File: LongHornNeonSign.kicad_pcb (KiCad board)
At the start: 2 copper layers, 68.1 x 76.2 mm, 19 parts, among them Q1 IRLZ44N, Q2 IRLZ44N, Q3 IRLZ44N

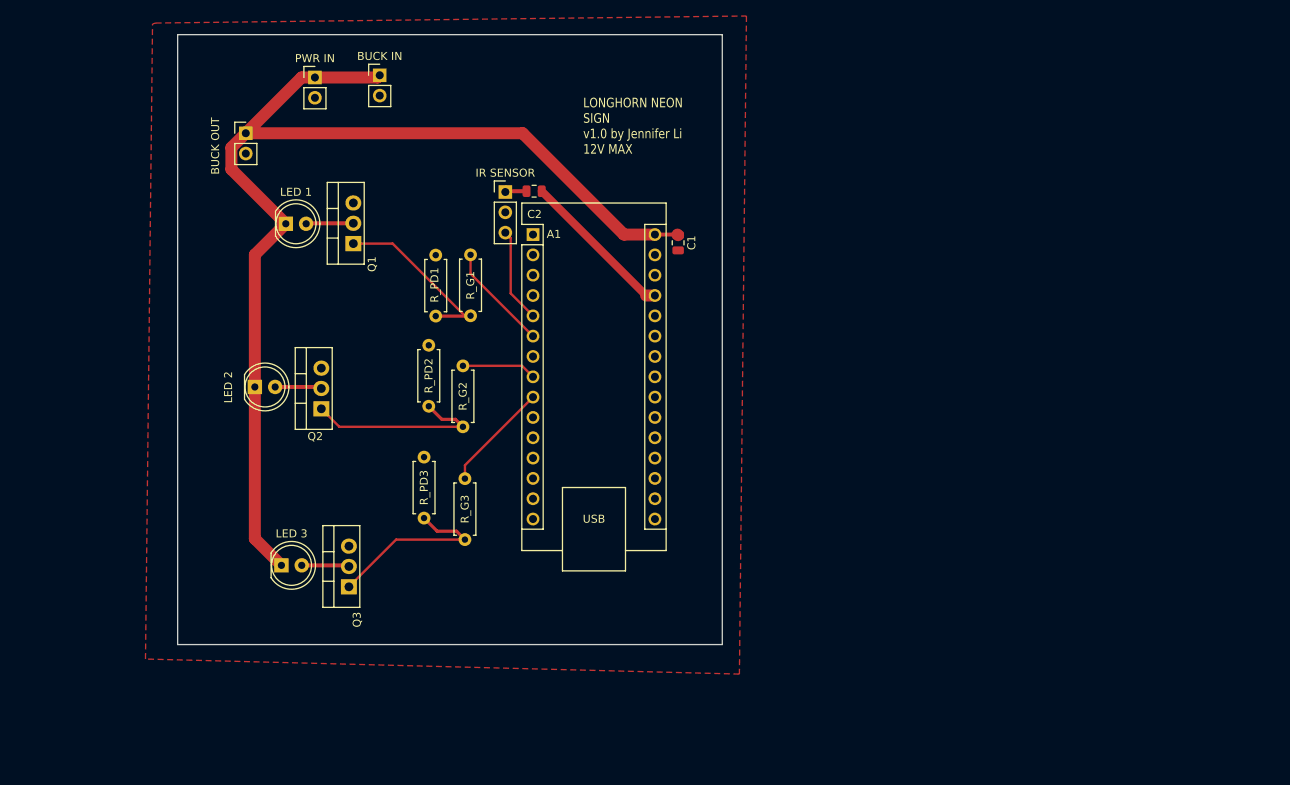
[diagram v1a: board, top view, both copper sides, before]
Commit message: update
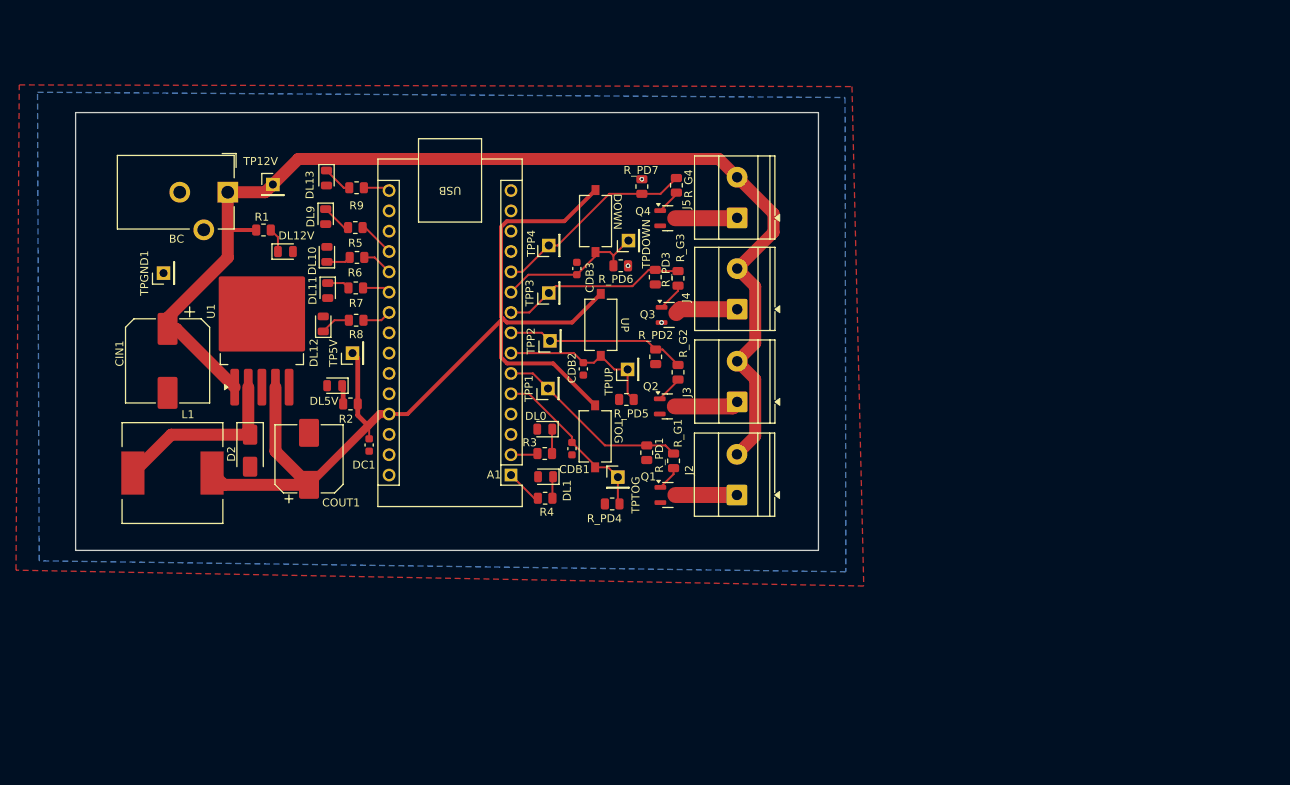
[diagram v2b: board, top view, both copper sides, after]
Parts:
- removed BUCK IN: Conn_01x02_Pin, Connector_PinHeader_2.54mm:PinHeader_1x02_P2.54mm_Vertical
- removed BUCK OUT: Conn_01x02_Pin, Connector_PinHeader_2.54mm:PinHeader_1x02_P2.54mm_Vertical
- removed C1, C2: 0.1uF, Capacitor_SMD:C_0805_2012Metric
- removed IR SENSOR: Conn_01x03, Connector_PinHeader_2.54mm:PinHeader_1x03_P2.54mm_Vertical
- removed LED 1: Conn_01x02_Pin, LED_THT:LED_D5.0mm
- removed LED 2: Conn_01x02_Pin, LED_THT:LED_D5.0mm
- removed LED 3: Conn_01x02_Pin, LED_THT:LED_D5.0mm
- removed PWR IN: Conn_01x02_Pin, Connector_PinHeader_2.54mm:PinHeader_1x02_P2.54mm_Vertical
- added BC: Barrel_Jack, Connector_BarrelJack:BarrelJack_CUI_PJ-102AH_Horizontal, F.Cu at (76.2, 71.6)
- added CDB1: 0.1uF, Capacitor_SMD:C_0603_1608Metric, F.Cu at (119.2, 103.7)
- added CDB2: 0.1uF, Capacitor_SMD:C_0603_1608Metric, F.Cu at (120.7, 93.7)
- added CDB3: 0.1uF, Capacitor_SMD:C_0603_1608Metric, F.Cu at (119.8, 81.2)
- added CIN1: 680μF, Capacitor_SMD:CP_Elec_10x10, F.Cu at (68.7, 92.7)
- added COUT1: 220μF, Capacitor_SMD:CP_Elec_8x10, F.Cu at (86.4, 105.0)
- added D2: SS34, Diode_SMD:D_SMA, F.Cu at (79.0, 103.9)
- added DC1: 0.1uF, Capacitor_SMD:C_0603_1608Metric, F.Cu at (93.9, 103.2)
- added DL0: DL_D0, LED_SMD:LED_0805_2012Metric, F.Cu at (115.8, 101.2)
- added DL1: DL_D1, LED_SMD:LED_0805_2012Metric, F.Cu at (115.9, 107.2)
- added DL10: DL_D10, LED_SMD:LED_0805_2012Metric, F.Cu at (88.6, 79.4)
- added DL11: DL_D11, LED_SMD:LED_0805_2012Metric, F.Cu at (88.7, 83.9)
- added DL12: DL_D12, LED_SMD:LED_0805_2012Metric, F.Cu at (88.1, 88.1)
- added DL12V: DL_12V, LED_SMD:LED_0805_2012Metric, F.Cu at (83.4, 79.0)
- added DL13: DL_D13, LED_SMD:LED_0805_2012Metric, F.Cu at (88.5, 69.8)
- added DL5V: DL_5V, LED_SMD:LED_0805_2012Metric, F.Cu at (89.6, 95.8)
- added DL9: DL_D9, LED_SMD:LED_0805_2012Metric, F.Cu at (88.4, 74.7)
- added DOWN: SW_Push, Button_Switch_SMD:SW_Tactile_SPST_NO_Straight_CK_PTS636Sx25SMTRLFS, F.Cu at (122.2, 75.2)
- added J2: Screw_Terminal_01x02, TerminalBlock_Phoenix:TerminalBlock_Phoenix_MKDS-1,5-2-5.08_1x02_P5.08mm_Horizontal, F.Cu at (139.9, 109.5)
- added J3: Screw_Terminal_01x02, TerminalBlock_Phoenix:TerminalBlock_Phoenix_MKDS-1,5-2-5.08_1x02_P5.08mm_Horizontal, F.Cu at (139.9, 97.8)
- added J4: Screw_Terminal_01x02, TerminalBlock_Phoenix:TerminalBlock_Phoenix_MKDS-1,5-2-5.08_1x02_P5.08mm_Horizontal, F.Cu at (139.9, 86.3)
- added J5: Screw_Terminal_01x02, TerminalBlock_Phoenix:TerminalBlock_Phoenix_MKDS-1,5-2-5.08_1x02_P5.08mm_Horizontal, F.Cu at (139.9, 74.8)
- added L1: 33μH, Inductor_SMD:L_12x12mm_H8mm, F.Cu at (69.3, 106.7)
- added Q4: AO3400A, Package_TO_SOT_SMD:SOT-23, F.Cu at (131.2, 74.9)
- added R1: 1kΩ, Resistor_SMD:R_0805_2012Metric, F.Cu at (80.7, 76.4)
- added R2: 470Ω, Resistor_SMD:R_0805_2012Metric, F.Cu at (91.5, 98.1)
- added R3: 470Ω, Resistor_SMD:R_0805_2012Metric, F.Cu at (115.8, 104.3)
- added R4: 470Ω, Resistor_SMD:R_0805_2012Metric, F.Cu at (115.9, 109.9)
- added R5: 470Ω, Resistor_SMD:R_0805_2012Metric, F.Cu at (92.1, 76.0)
- added R6: 470Ω, Resistor_SMD:R_0805_2012Metric, F.Cu at (92.4, 79.8)
- added R7: 470Ω, Resistor_SMD:R_0805_2012Metric, F.Cu at (92.2, 83.6)
- added R8: 470Ω, Resistor_SMD:R_0805_2012Metric, F.Cu at (92.3, 87.6)
- added R9: 470Ω, Resistor_SMD:R_0805_2012Metric, F.Cu at (92.3, 71.1)
- added R_G4: 220, Resistor_SMD:R_0805_2012Metric, F.Cu at (132.3, 70.8)
- added R_PD4: 10kΩ, Resistor_SMD:R_0805_2012Metric, F.Cu at (124.3, 110.6)
- added R_PD5: 10kΩ, Resistor_SMD:R_0805_2012Metric, F.Cu at (126.0, 97.5)
- added R_PD6: 10kΩ, Resistor_SMD:R_0805_2012Metric, F.Cu at (125.3, 80.8)
- added R_PD7: 10kΩ, Resistor_SMD:R_0805_2012Metric, F.Cu at (128.0, 70.9)
- added TOG: SW_Push, Button_Switch_SMD:SW_Tactile_SPST_NO_Straight_CK_PTS636Sx25SMTRLFS, F.Cu at (122.1, 102.1)
- added TP12V: +12V, Connector_PinHeader_2.54mm:PinHeader_1x01_P2.54mm_Vertical, F.Cu at (81.8, 70.7)
- added TP5V: +5V, Connector_PinHeader_2.54mm:PinHeader_1x01_P2.54mm_Vertical, F.Cu at (91.8, 91.7)
- added TPDOWN: BTN_DOWN, Connector_PinHeader_2.54mm:PinHeader_1x01_P2.54mm_Vertical, F.Cu at (126.3, 77.7)
- added TPGND1: GND, Connector_PinHeader_2.54mm:PinHeader_1x01_P2.54mm_Vertical, F.Cu at (68.2, 81.7)
- added TPP1: PWM_OUT1, Connector_PinHeader_2.54mm:PinHeader_1x01_P2.54mm_Vertical, F.Cu at (116.2, 96.2)
- added TPP2: PWM_OUT2, Connector_PinHeader_2.54mm:PinHeader_1x01_P2.54mm_Vertical, F.Cu at (116.5, 90.2)
- added TPP3: PWM_OUT3, Connector_PinHeader_2.54mm:PinHeader_1x01_P2.54mm_Vertical, F.Cu at (116.3, 84.2)
- added TPP4: PWM_OUT4, Connector_PinHeader_2.54mm:PinHeader_1x01_P2.54mm_Vertical, F.Cu at (116.3, 78.3)
- added TPTOG: BTN_TOGGLE, Connector_PinHeader_2.54mm:PinHeader_1x01_P2.54mm_Vertical, F.Cu at (125.0, 107.2)
- added TPUP: BTN_UP, Connector_PinHeader_2.54mm:PinHeader_1x01_P2.54mm_Vertical, F.Cu at (126.2, 93.8)
- added U1: LM2596S-5, Package_TO_SOT_SMD:TO-263-5_TabPin3, F.Cu at (80.5, 88.3)
- added UP: SW_Push, Button_Switch_SMD:SW_Tactile_SPST_NO_Straight_CK_PTS636Sx25SMTRLFS, F.Cu at (122.8, 88.2)
- A1: value Metro Mini 328 Stand in -> Arduino Nano
- Q1, Q2, Q3: value IRLZ44N -> AO3400A; footprint Package_TO_SOT_THT:TO-220-3_Vertical -> Package_TO_SOT_SMD:SOT-23
- R_G1, R_G2, R_G3: footprint Resistor_THT:R_Axial_DIN0207_L6.3mm_D2.5mm_P7.62mm_Horizontal -> Resistor_SMD:R_0805_2012Metric
- R_PD1, R_PD2, R_PD3: value 10k -> 10kΩ; footprint Resistor_THT:R_Axial_DIN0207_L6.3mm_D2.5mm_P7.62mm_Horizontal -> Resistor_SMD:R_0805_2012Metric
- moved Q3 52.5 mm to (131.4, 87.0), turned to 0 degrees
- moved Q1 50.3 mm to (131.2, 109.5), turned to 0 degrees
- moved Q2 43.2 mm to (131.1, 98.4), turned to 0 degrees
- moved R_G3 42.1 mm to (132.5, 82.4), turned to -90 degrees
- moved R_PD3 41.7 mm to (129.6, 82.2), turned to -90 degrees
- moved R_PD1 31.4 mm to (128.6, 104.2), turned to -90 degrees
- moved R_G1 31.2 mm to (131.9, 105.2), turned to -90 degrees
- moved A1 30.2 mm to (111.6, 107.0), turned to 180 degrees
- moved R_PD2 28.4 mm to (129.7, 92.2)
- moved R_G2 27.7 mm to (132.5, 94.1), turned to -90 degrees
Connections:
- A1 pad 1: unconnected-(A1-D1/TX-Pad1) -> /D_DEBUG1
- A1 pad 10: unconnected-(A1-D7-Pad10) -> /BTN_DOWN
- A1 pad 11: unconnected-(A1-D8-Pad11) -> /PWM_OUT4
- A1 pad 16: unconnected-(A1-D13-Pad16) -> /D_DEBUG13
- A1 pad 19: unconnected-(A1-A0-Pad19) -> /D_DEBUG9
- A1 pad 2: unconnected-(A1-D0/RX-Pad2) -> /D_DEBUG0
- A1 pad 20: unconnected-(A1-A1-Pad20) -> /D_DEBUG10
- A1 pad 21: unconnected-(A1-A2-Pad21) -> /D_DEBUG11
- A1 pad 22: unconnected-(A1-A3-Pad22) -> /D_DEBUG12
- A1 pad 27: Net-(A1-+5V) -> /+5V
- A1 pad 30: /+12V  -> unconnected-(A1-VIN-Pad30)
- A1 pad 5: /OUT -> /BTN_TOGGLE
- A1 pad 7: unconnected-(A1-D4-Pad7) -> /BTN_UP
- Q1 pad 2: Net-(LED_OUT1-Pin_2) -> GND
- Q1 pad 3: GND -> Net-(J2-Pin_1)
- Q2 pad 2: Net-(LED_OUT2-Pin_2) -> GND
- Q2 pad 3: GND -> Net-(J3-Pin_1)
- Q3 pad 2: Net-(LED_OUT3-Pin_2) -> GND
- Q3 pad 3: GND -> Net-(J4-Pin_1)
- R_G1 pad 1: Net-(Q1-G) -> /PWM_OUT1
- R_G1 pad 2: /PWM_OUT1 -> Net-(Q1-G)
- R_G2 pad 1: Net-(Q2-G) -> /PWM_OUT2
- R_G2 pad 2: /PWM_OUT2 -> Net-(Q2-G)
- R_G3 pad 1: Net-(Q3-G) -> /PWM_OUT3
- R_G3 pad 2: /PWM_OUT3 -> Net-(Q3-G)
- R_PD1 pad 1: Net-(Q1-G) -> /PWM_OUT1
- R_PD2 pad 1: GND -> /PWM_OUT2
- R_PD2 pad 2: Net-(Q2-G) -> GND
- R_PD3 pad 1: Net-(Q3-G) -> /PWM_OUT3
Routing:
- net +12V: track 0.00 -> 143.7 mm
- net /+12V : track 139.6 -> 0.00 mm
- net /+5V: track 0.00 -> 129.5 mm
- net /PWM_OUT4: track 0.00 -> 25.5 mm
- net Net-(D2-K): track 0.00 -> 22.7 mm
- net /BTN_TOGGLE: track 0.00 -> 21.7 mm
- net Net-(Q2-G): track 24.0 -> 3.35 mm
- net /BTN_UP: track 0.00 -> 20.2 mm
- net /BTN_DOWN: track 0.00 -> 19.8 mm
- net Net-(Q1-G): track 22.8 -> 3.09 mm
- net Net-(Q3-G): track 23.2 -> 3.56 mm
- net Net-(A1-+5V): track 19.6 -> 0.00 mm
- net /PWM_OUT2: track 9.33 -> 22.5 mm
- net /OUT: track 11.8 -> 0.00 mm
- net /PWM_OUT1: track 13.4 -> 24.5 mm
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- added copper zone on B.Cu, net GND
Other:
- board size 68.1 x 76.2 mm -> 92.9 x 54.7 mm
- board text removed: "LONGHORN NEON SIGN v1.0 by Jennifer Li 12V MAX"

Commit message: update
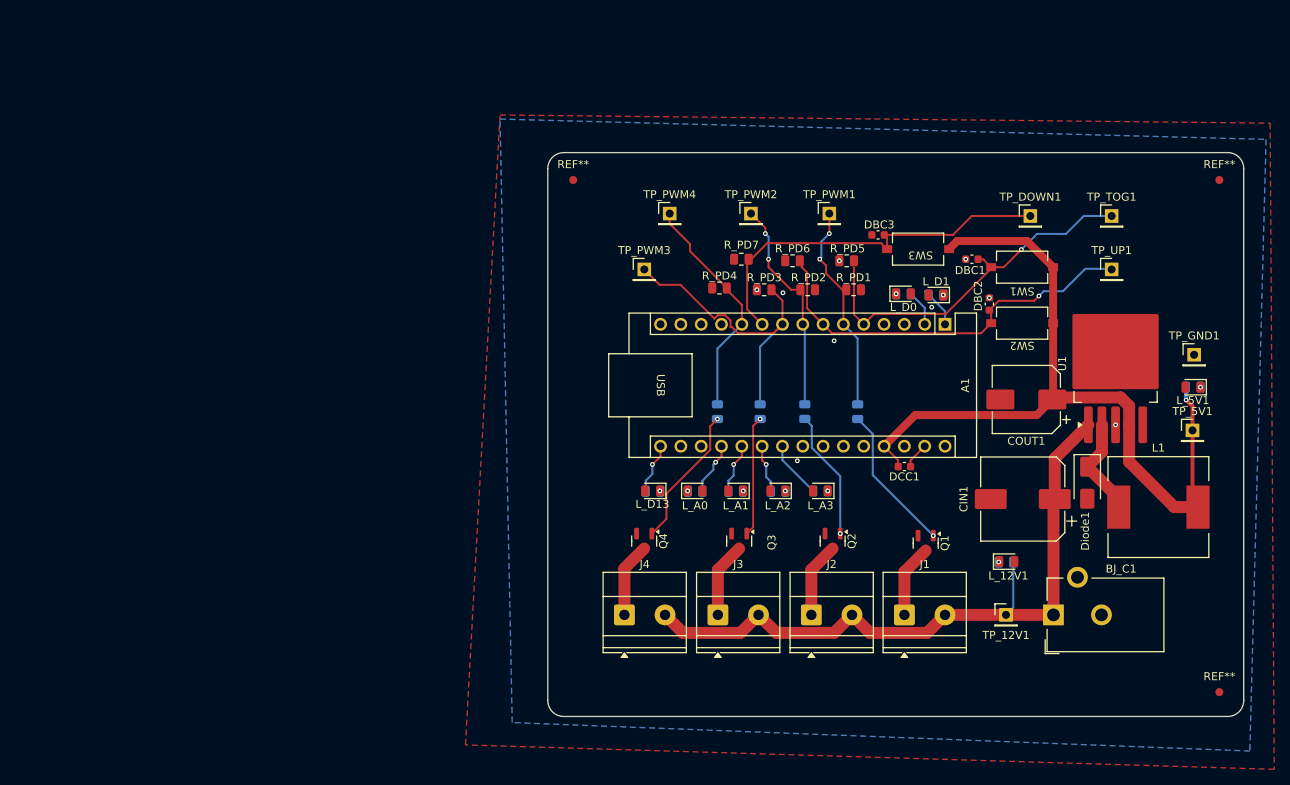
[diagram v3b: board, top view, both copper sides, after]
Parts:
- removed BC: Barrel_Jack, Connector_BarrelJack:BarrelJack_CUI_PJ-102AH_Horizontal
- removed CDB1, CDB2, CDB3, DC1: 0.1uF, Capacitor_SMD:C_0603_1608Metric
- removed D2: SS34, Diode_SMD:D_SMA
- removed DL0: DL_D0, LED_SMD:LED_0805_2012Metric
- removed DL1: DL_D1, LED_SMD:LED_0805_2012Metric
- removed DL10: DL_D10, LED_SMD:LED_0805_2012Metric
- removed DL11: DL_D11, LED_SMD:LED_0805_2012Metric
- removed DL12: DL_D12, LED_SMD:LED_0805_2012Metric
- removed DL12V: DL_12V, LED_SMD:LED_0805_2012Metric
- removed DL13: DL_D13, LED_SMD:LED_0805_2012Metric
- removed DL5V: DL_5V, LED_SMD:LED_0805_2012Metric
- removed DL9: DL_D9, LED_SMD:LED_0805_2012Metric
- removed DOWN, TOG, UP: SW_Push, Button_Switch_SMD:SW_Tactile_SPST_NO_Straight_CK_PTS636Sx25SMTRLFS
- removed J5: Screw_Terminal_01x02, TerminalBlock_Phoenix:TerminalBlock_Phoenix_MKDS-1,5-2-5.08_1x02_P5.08mm_Horizontal
- removed R1: 1kΩ, Resistor_SMD:R_0805_2012Metric
- removed R2, R3, R4, R5, R6, R7, R8, R9: 470Ω, Resistor_SMD:R_0805_2012Metric
- removed TP12V: +12V, Connector_PinHeader_2.54mm:PinHeader_1x01_P2.54mm_Vertical
- removed TP5V: +5V, Connector_PinHeader_2.54mm:PinHeader_1x01_P2.54mm_Vertical
- removed TPDOWN: BTN_DOWN, Connector_PinHeader_2.54mm:PinHeader_1x01_P2.54mm_Vertical
- removed TPGND1: GND, Connector_PinHeader_2.54mm:PinHeader_1x01_P2.54mm_Vertical
- removed TPP1: PWM_OUT1, Connector_PinHeader_2.54mm:PinHeader_1x01_P2.54mm_Vertical
- removed TPP2: PWM_OUT2, Connector_PinHeader_2.54mm:PinHeader_1x01_P2.54mm_Vertical
- removed TPP3: PWM_OUT3, Connector_PinHeader_2.54mm:PinHeader_1x01_P2.54mm_Vertical
- removed TPP4: PWM_OUT4, Connector_PinHeader_2.54mm:PinHeader_1x01_P2.54mm_Vertical
- removed TPTOG: BTN_TOGGLE, Connector_PinHeader_2.54mm:PinHeader_1x01_P2.54mm_Vertical
- removed TPUP: BTN_UP, Connector_PinHeader_2.54mm:PinHeader_1x01_P2.54mm_Vertical
- added BJ_C1: Barrel_Jack, Connector_BarrelJack:BarrelJack_CUI_PJ-102AH_Horizontal, F.Cu at (179.4, 124.5)
- added DBC1: 0.1uF, Capacitor_SMD:C_0603_1608Metric, F.Cu at (169.2, 80.0)
- added DBC2: 0.1uF, Capacitor_SMD:C_0603_1608Metric, F.Cu at (171.4, 85.6)
- added DBC3: 0.1uF, Capacitor_SMD:C_0603_1608Metric, F.Cu at (157.5, 77.0)
- added DCC1: 0.1uF, Capacitor_SMD:C_0603_1608Metric, F.Cu at (160.8, 105.9)
- added Diode1: SS34, Diode_SMD:D_SMA, F.Cu at (183.6, 107.9)
- added J1: Screw_Terminal_01x02, TerminalBlock_Phoenix:TerminalBlock_Phoenix_MKDS-1,5-2-5.08_1x02_P5.08mm_Horizontal, F.Cu at (160.8, 124.5)
- added L_12V1: 12V, LED_SMD:LED_0805_2012Metric, F.Cu at (173.6, 117.8)
- added L_5V1: 5V, LED_SMD:LED_0805_2012Metric, F.Cu at (196.8, 96.0)
- added L_A0: A0, LED_SMD:LED_0805_2012Metric, F.Cu at (134.6, 109.0)
- added L_A1: A1, LED_SMD:LED_0805_2012Metric, F.Cu at (139.7, 109.0)
- added L_A2: A2, LED_SMD:LED_0805_2012Metric, F.Cu at (145.0, 109.0)
- added L_A3: A3, LED_SMD:LED_0805_2012Metric, F.Cu at (150.3, 109.0)
- added L_D0: D0, LED_SMD:LED_0805_2012Metric, F.Cu at (160.7, 84.3)
- added L_D1: D1, LED_SMD:LED_0805_2012Metric, F.Cu at (164.7, 84.5)
- added L_D13: D13, LED_SMD:LED_0805_2012Metric, F.Cu at (129.3, 109.0)
- added REF**: Fiducial_1mm_Mask2mm, Fiducial:Fiducial_1mm_Mask2mm, F.Cu at (200.2, 70.1)
- added REF**: Fiducial_1mm_Mask2mm, Fiducial:Fiducial_1mm_Mask2mm, F.Cu at (200.2, 134.1)
- added REF**: Fiducial_1mm_Mask2mm, Fiducial:Fiducial_1mm_Mask2mm, F.Cu at (119.4, 70.1)
- added R_12V1: 1kΩ, Resistor_SMD:R_0805_2012Metric, B.Cu at (173.5, 117.9)
- added R_5V1: 470Ω, Resistor_SMD:R_0805_2012Metric, B.Cu at (196.9, 96.0)
- added R_A0: 470Ω, Resistor_SMD:R_0805_2012Metric, B.Cu at (134.6, 109.0)
- added R_A1: 470Ω, Resistor_SMD:R_0805_2012Metric, B.Cu at (139.7, 109.0)
- added R_A2: 470Ω, Resistor_SMD:R_0805_2012Metric, B.Cu at (145.0, 109.0)
- added R_A3: 470Ω, Resistor_SMD:R_0805_2012Metric, B.Cu at (150.3, 109.0)
- added R_D0: 470Ω, Resistor_SMD:R_0805_2012Metric, B.Cu at (160.7, 84.3)
- added R_D1: 470Ω, Resistor_SMD:R_0805_2012Metric, B.Cu at (164.7, 84.5)
- added R_D13: 470Ω, Resistor_SMD:R_0805_2012Metric, B.Cu at (129.4, 109.0)
- added SW1: SW_Push, Button_Switch_SMD:SW_Tactile_SPST_NO_Straight_CK_PTS636Sx25SMTRLFS, F.Cu at (175.5, 81.0)
- added SW2: SW_Push, Button_Switch_SMD:SW_Tactile_SPST_NO_Straight_CK_PTS636Sx25SMTRLFS, F.Cu at (175.5, 88.0)
- added SW3: SW_Push, Button_Switch_SMD:SW_Tactile_SPST_NO_Straight_CK_PTS636Sx25SMTRLFS, F.Cu at (162.5, 78.7)
- added TP_12V1: +12V, Connector_PinHeader_2.54mm:PinHeader_1x01_P2.54mm_Vertical, F.Cu at (173.5, 124.5)
- added TP_5V1: +5V, Connector_PinHeader_2.54mm:PinHeader_1x01_P2.54mm_Vertical, F.Cu at (196.8, 101.4)
- added TP_DOWN1: DOWN, Connector_PinHeader_2.54mm:PinHeader_1x01_P2.54mm_Vertical, F.Cu at (176.5, 74.6)
- added TP_GND1: GND, Connector_PinHeader_2.54mm:PinHeader_1x01_P2.54mm_Vertical, F.Cu at (197.0, 91.9)
- added TP_PWM1: PWM1, Connector_PinHeader_2.54mm:PinHeader_1x01_P2.54mm_Vertical, F.Cu at (151.4, 74.3)
- added TP_PWM2: PWM2, Connector_PinHeader_2.54mm:PinHeader_1x01_P2.54mm_Vertical, F.Cu at (141.6, 74.3)
- added TP_PWM3: PWM3, Connector_PinHeader_2.54mm:PinHeader_1x01_P2.54mm_Vertical, F.Cu at (128.3, 81.3)
- added TP_PWM4: PWM4, Connector_PinHeader_2.54mm:PinHeader_1x01_P2.54mm_Vertical, F.Cu at (131.4, 74.3)
- added TP_TOG1: TOGGLE, Connector_PinHeader_2.54mm:PinHeader_1x01_P2.54mm_Vertical, F.Cu at (186.7, 74.6)
- added TP_UP1: UP, Connector_PinHeader_2.54mm:PinHeader_1x01_P2.54mm_Vertical, F.Cu at (186.7, 81.3)
- R_G1, R_G2, R_G3, R_G4: moved to B.Cu
- moved L1 123.3 mm to (192.5, 111.0)
- moved CIN1 108.3 mm to (175.6, 110.0), turned to 180 degrees
- moved U1 106.8 mm to (187.2, 93.1)
- moved COUT1 90.0 mm to (176.0, 97.5), turned to 180 degrees
- moved A1 57.4 mm to (165.9, 88.1), turned to -90 degrees
- moved J4 40.7 mm to (125.8, 124.5), turned to 0 degrees
- moved Q4 40.5 mm to (128.3, 115.2), turned to -90 degrees
- moved R_PD1 32.9 mm to (154.4, 83.8), turned to 0 degrees
- moved Q1 32.8 mm to (163.4, 115.5), turned to -90 degrees
- moved R_PD5 32.5 mm to (153.6, 80.2)
- moved R_PD4 30.1 mm to (137.7, 83.6)
- moved Q3 29.6 mm to (140.1, 115.2), turned to -90 degrees
- moved R_G4 28.8 mm to (137.4, 99.1)
- moved J3 26.7 mm to (137.5, 124.5), turned to 0 degrees
- moved Q2 26.7 mm to (151.8, 115.2), turned to -90 degrees
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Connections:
- net /PWM_OUT1 renamed /PWM1
- net /PWM_OUT2 renamed /PWM2
- net /PWM_OUT3 renamed /PWM3
- A1 pad 1: /D_DEBUG1 -> /D_D1
- A1 pad 10: /BTN_DOWN -> /DOWN
- A1 pad 11: /PWM_OUT4 -> /PWM4
- A1 pad 16: /D_DEBUG13 -> /D_D13
- A1 pad 19: /D_DEBUG9 -> /D_A0
- A1 pad 2: /D_DEBUG0 -> /D_D0
- A1 pad 20: /D_DEBUG10 -> /D_A1
- A1 pad 21: /D_DEBUG11 -> /D_A2
- A1 pad 22: /D_DEBUG12 -> /D_A3
- A1 pad 5: /BTN_TOGGLE -> /TOG
- A1 pad 7: /BTN_UP -> /UP
- Q1 pad 3: Net-(J2-Pin_1) -> Net-(J1-Pin_1)
- Q2 pad 3: Net-(J3-Pin_1) -> Net-(J2-Pin_1)
- Q3 pad 3: Net-(J4-Pin_1) -> Net-(J3-Pin_1)
- Q4 pad 3: Net-(J5-Pin_1) -> Net-(J4-Pin_1)
- R_G4 pad 1: /PWM_OUT4 -> /PWM4
- R_PD4 pad 1: /BTN_TOGGLE -> /PWM4
- R_PD5 pad 1: /BTN_UP -> /TOG
- R_PD6 pad 1: /BTN_DOWN -> /UP
- R_PD7 pad 1: /PWM_OUT4 -> /DOWN
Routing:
- net +12V: track 143.7 -> 86.7 mm
- net /UP: track 0.00 -> 50.0 mm, vias 0 -> 1
- net /DOWN: track 0.00 -> 48.6 mm
- net /TOG: track 0.00 -> 46.6 mm, vias 0 -> 1
- net /PWM4: track 0.00 -> 28.8 mm
- net /+5V: track 129.5 -> 101.8 mm, vias 0 -> 1
- net /PWM_OUT4: track 25.5 -> 0.00 mm
- net /BTN_TOGGLE: track 21.7 -> 0.00 mm
- net /BTN_UP: track 20.2 -> 0.00 mm
- net /BTN_DOWN: track 19.8 -> 0.00 mm
- net Net-(Q1-G): track 3.09 -> 18.5 mm, vias 0 -> 1
- net /PWM3: track 23.1 -> 37.9 mm
- net Net-(Q4-G): track 3.31 -> 17.7 mm, vias 0 -> 1
- net Net-(Q2-G): track 3.35 -> 16.2 mm, vias 0 -> 1
- net Net-(Q3-G): track 3.56 -> 15.0 mm, vias 0 -> 1
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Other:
- board size 92.9 x 54.7 mm -> 87 x 70.5 mm
